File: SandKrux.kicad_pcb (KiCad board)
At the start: 2 copper layers, 4 parts, among them U1 K210_C913414, U2 AXP173, U3 MT9700-N, U4 SGM809-ZXN3L/TR

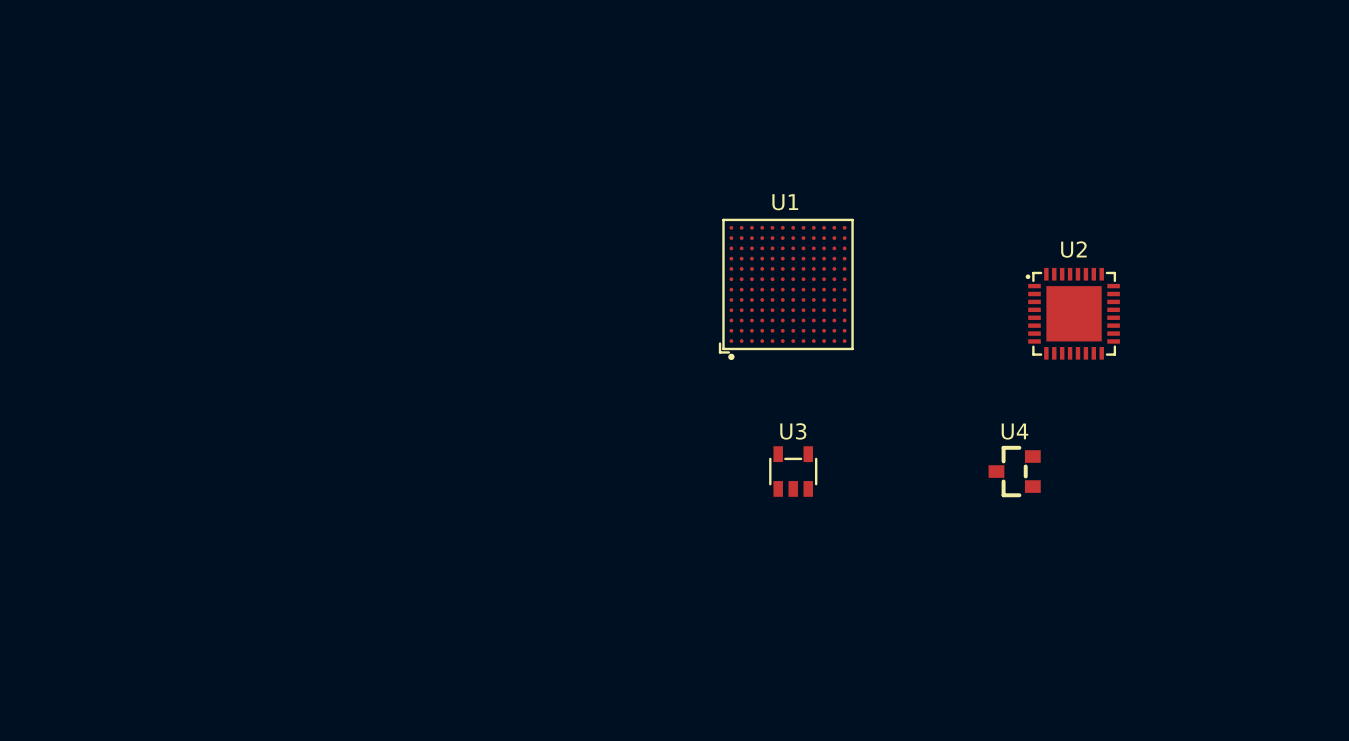
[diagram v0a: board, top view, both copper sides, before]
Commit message: K210 E SISTEMAS DE ENERGIA DO MODULO PRINCIPAL
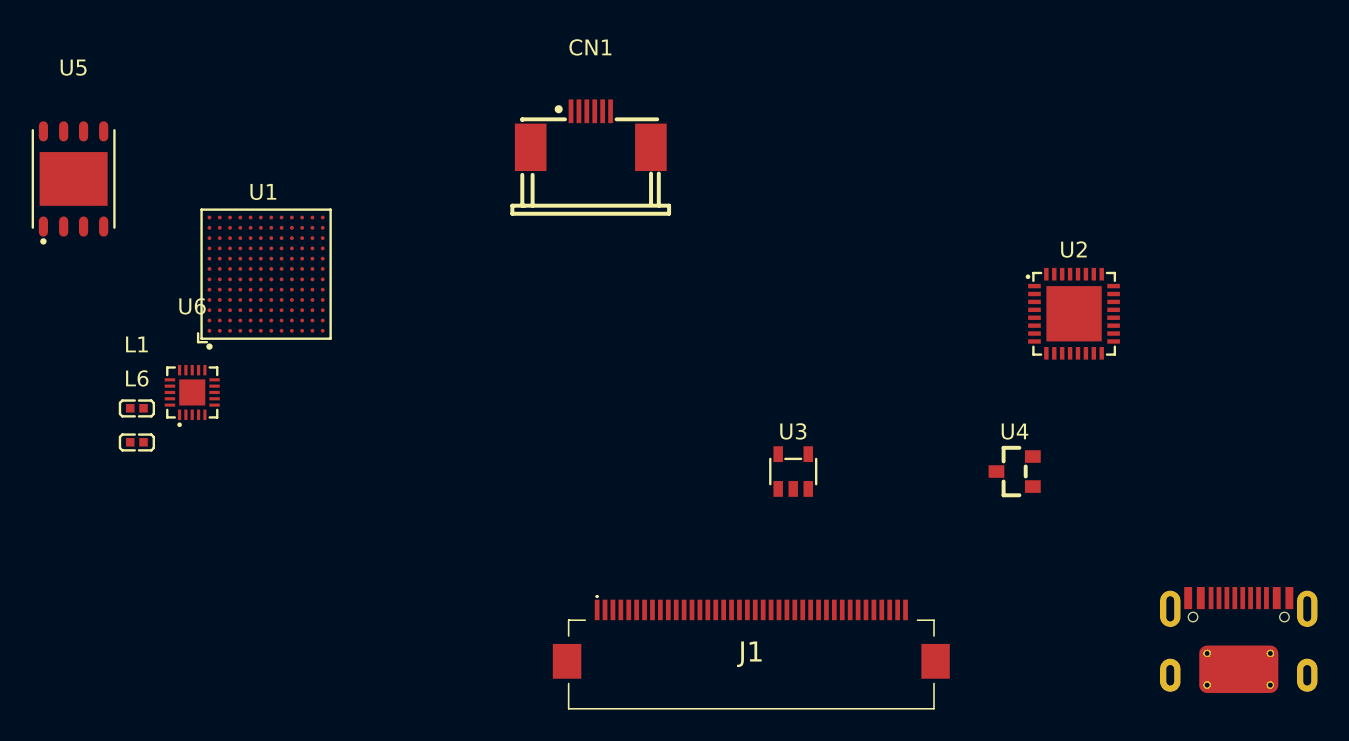
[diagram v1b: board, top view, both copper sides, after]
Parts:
- added CN1: 527450697, easyeda2kicad:CONN-SMD_527450697, F.Cu at (113.2, 67.9)
- added J1: FH12-40S-0.5SH_55_, KiCad:FH1240S05SH55, F.Cu at (123.3, 100.9)
- added J2: Connector, USB-TYPE-C-16P, PCM_JLCPCB:TYPE-C-SMD_HX-TYPE-C-16PIN, F.Cu at (154.2, 100.0)
- added L1: CBW100505U601T, easyeda2kicad:L0402, F.Cu at (84.5, 85.5)
- added L6: CBW100505U601T, easyeda2kicad:L0402, F.Cu at (84.5, 87.7)
- added U5: GD25LQ128EWIGR, easyeda2kicad:WSON-8_L6.0-W5.0-P1.27-BL-EP, F.Cu at (80.5, 71.0)
- added U6: TMI7003C, easyeda2kicad:QFN-20_L3.0-W3.0-P0.40-BL-EP1.7, F.Cu at (88.0, 84.5)
- moved U1 33.0 mm to (92.7, 77.0)
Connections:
- U1 pad C3: unconnected-(U1-VSS-PadC3) -> GND
- U1 pad C5: unconnected-(U1-VDDIO5B-PadC5) -> /<NO NET>
